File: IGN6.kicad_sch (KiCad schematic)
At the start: 6 parts

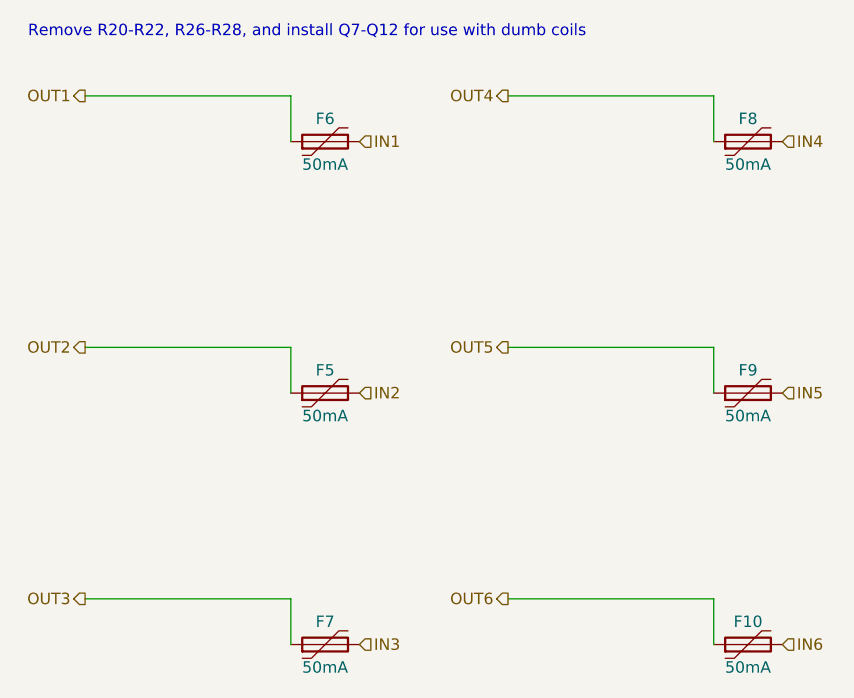
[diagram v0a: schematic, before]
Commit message: test
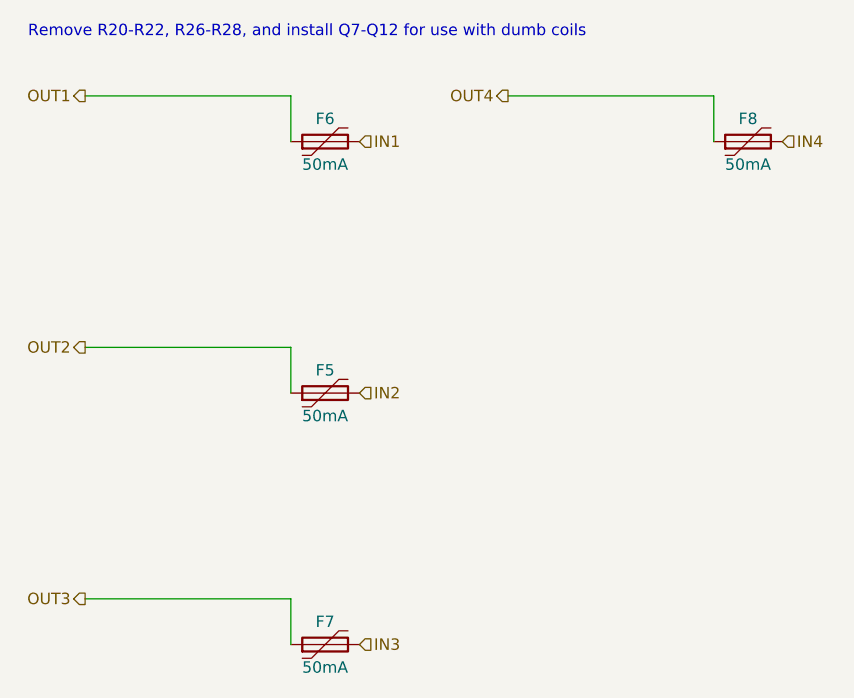
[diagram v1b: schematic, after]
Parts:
- removed F10, F9: 50mA, Fuse:Fuse_0603_1608Metric, symbol Device:Polyfuse
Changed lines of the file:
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@@
-	(wire
-		(pts
-			(xy 160.02 120.65) (xy 182.88 120.65)
-		)
-		(stroke
-			(width 0)
-			(type default)
-		)
-	)
 	(wire
 		(pts
@@
 		(pts
 			(xy 113.03 92.71) (xy 135.89 92.71)
-		)
-		(stroke
-			(width 0)
-			(type default)
-		)
-	)
-	(wire
-		(pts
-			(xy 160.02 92.71) (xy 182.88 92.71)
-		)
-		(stroke
-			(width 0)
-			(type default)
-		)
-	)
-	(wire
-		(pts
-			(xy 182.88 92.71) (xy 182.88 97.79)
-		)
-		(stroke
-			(width 0)
-			(type default)
-		)
-	)
-	(wire
-		(pts
-			(xy 182.88 120.65) (xy 182.88 125.73)
 		)
 		(stroke
@@
 			)
 			(justify left bottom)
-		)
-	)
-	(hierarchical_label "IN5"
-		(shape input)
-		(at 190.5 97.79 0)
-		(fields_autoplaced yes)
-		(effects
-			(font
-				(size 1.27 1.27)
-			)
-			(justify left)
 		)
 	)
@@
 			)
 			(justify left)
-		)
-	)
-	(hierarchical_label "IN6"
-		(shape input)
-		(at 190.5 125.73 0)
-		(fields_autoplaced yes)
-		(effects
-			(font
-				(size 1.27 1.27)
-			)
-			(justify left)
-		)
-	)
-	(hierarchical_label "OUT6"
-		(shape output)
-		(at 160.02 120.65 180)
-		(fields_autoplaced yes)
-		(effects
-			(font
-				(size 1.27 1.27)
-			)
-			(justify right)
-		)
-	)
-	(hierarchical_label "OUT5"
-		(shape output)
-		(at 160.02 92.71 180)
-		(fields_autoplaced yes)
-		(effects
-			(font
-				(size 1.27 1.27)
-			)
-			(justify right)
 		)
 	)
@@
 		)
 	)
-	(symbol
-		(lib_id "Device:Polyfuse")
-		(at 186.69 125.73 90)
-		(unit 1)
-		(exclude_from_sim no)
-		(in_bom yes)
-		(on_board yes)
-		(dnp no)
-		(property "Reference" "F10"
-			(at 186.69 123.19 90)
-			(effects
-				(font
-					(size 1.27 1.27)
-				)
-			)
-		)
-		(property "Value" "50mA"
-			(at 186.69 128.27 90)
-			(effects
-				(font
-					(size 1.27 1.27)
-				)
-			)
-		)
-		(property "Footprint" "Fuse:Fuse_0603_1608Metric"
-			(at 191.77 124.46 0)
-			(effects
-				(font
-					(size 1.27 1.27)
-				)
-				(justify left)
-				(hide yes)
-			)
-		)
-		(property "Datasheet" "~"
-			(at 186.69 125.73 0)
-			(effects
-				(font
-					(size 1.27 1.27)
-				)
-				(hide yes)
-			)
-		)
-		(property "Description" ""
-			(at 186.69 125.73 0)
-			(effects
-				(font
-					(size 1.27 1.27)
-				)
-				(hide yes)
-			)
-		)
-		(property "LCSC" "C369141"
-			(at 186.69 125.73 90)
-			(effects
-				(font
-					(size 1.27 1.27)
-				)
-				(hide yes)
-			)
-		)
-		(pin "1"
-		)
-		(pin "2"
-		)
-		(instances
-			(project "uaefi"
-				(path "/ac264c30-3e9a-4be2-b97a-9949b68bd497/92c4206f-a69e-4d4d-9308-206d3518e11e"
-					(reference "F10")
-					(unit 1)
-				)
-			)
-		)
-	)
-	(symbol
-		(lib_id "Device:Polyfuse")
-		(at 186.69 97.79 90)
-		(unit 1)
-		(exclude_from_sim no)
-		(in_bom yes)
-		(on_board yes)
-		(dnp no)
-		(property "Reference" "F9"
-			(at 186.69 95.25 90)
-			(effects
-				(font
-					(size 1.27 1.27)
-				)
-			)
-		)
-		(property "Value" "50mA"
-			(at 186.69 100.33 90)
-			(effects
-				(font
-					(size 1.27 1.27)
-				)
-			)
-		)
-		(property "Footprint" "Fuse:Fuse_0603_1608Metric"
-			(at 191.77 96.52 0)
-			(effects
-				(font
-					(size 1.27 1.27)
-				)
-				(justify left)
-				(hide yes)
-			)
-		)
-		(property "Datasheet" "~"
-			(at 186.69 97.79 0)
-			(effects
-				(font
-					(size 1.27 1.27)
-				)
-				(hide yes)
-			)
-		)
-		(property "Description" ""
-			(at 186.69 97.79 0)
-			(effects
-				(font
-					(size 1.27 1.27)
-				)
-				(hide yes)
-			)
-		)
-		(property "LCSC" "C369141"
-			(at 186.69 97.79 90)
-			(effects
-				(font
-					(size 1.27 1.27)
-				)
-				(hide yes)
-			)
-		)
-		(pin "1"
-		)
-		(pin "2"
-		)
-		(instances
-			(project "uaefi"
-				(path "/ac264c30-3e9a-4be2-b97a-9949b68bd497/92c4206f-a69e-4d4d-9308-206d3518e11e"
-					(reference "F9")
-					(unit 1)
-				)
-			)
-		)
-	)

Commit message: reset
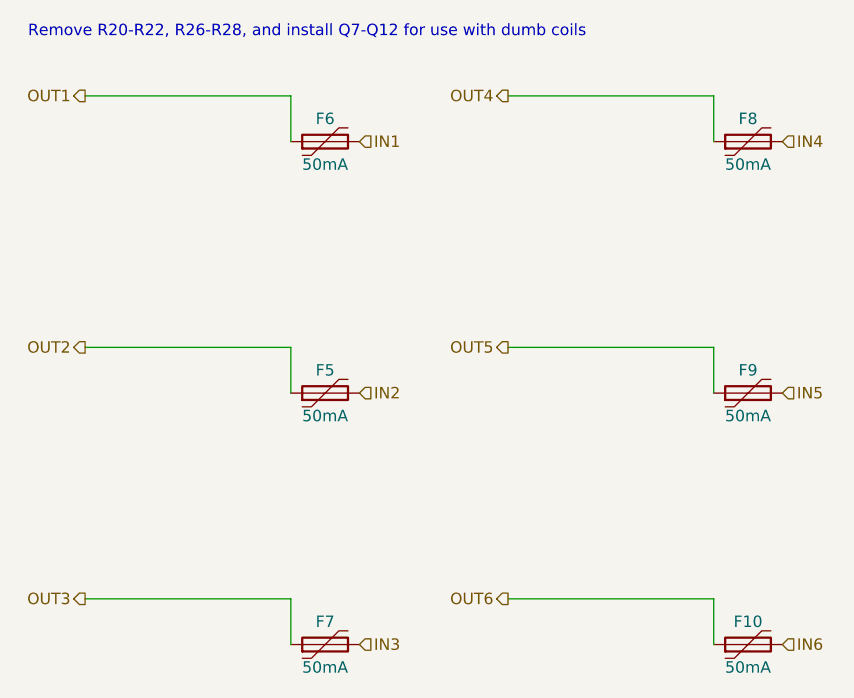
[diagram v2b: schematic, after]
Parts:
- added F10, F9: 50mA, Fuse:Fuse_0603_1608Metric, symbol Device:Polyfuse
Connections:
- new net IN5: F9.2
- new net IN6: F10.2
- new net OUT5: F9.1
- new net OUT6: F10.1
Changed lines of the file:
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@@
+	(wire
+		(pts
+			(xy 160.02 120.65) (xy 182.88 120.65)
+		)
+		(stroke
+			(width 0)
+			(type default)
+		)
+	)
 	(wire
 		(pts
@@
 		(pts
 			(xy 113.03 92.71) (xy 135.89 92.71)
+		)
+		(stroke
+			(width 0)
+			(type default)
+		)
+	)
+	(wire
+		(pts
+			(xy 160.02 92.71) (xy 182.88 92.71)
+		)
+		(stroke
+			(width 0)
+			(type default)
+		)
+	)
+	(wire
+		(pts
+			(xy 182.88 92.71) (xy 182.88 97.79)
+		)
+		(stroke
+			(width 0)
+			(type default)
+		)
+	)
+	(wire
+		(pts
+			(xy 182.88 120.65) (xy 182.88 125.73)
 		)
 		(stroke
@@
 		)
 	)
+	(hierarchical_label "IN5"
+		(shape input)
+		(at 190.5 97.79 0)
+		(fields_autoplaced yes)
+		(effects
+			(font
+				(size 1.27 1.27)
+			)
+			(justify left)
+		)
+	)
 	(hierarchical_label "OUT1"
 		(shape output)
@@
 		)
 	)
+	(hierarchical_label "IN6"
+		(shape input)
+		(at 190.5 125.73 0)
+		(fields_autoplaced yes)
+		(effects
+			(font
+				(size 1.27 1.27)
+			)
+			(justify left)
+		)
+	)
+	(hierarchical_label "OUT6"
+		(shape output)
+		(at 160.02 120.65 180)
+		(fields_autoplaced yes)
+		(effects
+			(font
+				(size 1.27 1.27)
+			)
+			(justify right)
+		)
+	)
+	(hierarchical_label "OUT5"
+		(shape output)
+		(at 160.02 92.71 180)
+		(fields_autoplaced yes)
+		(effects
+			(font
+				(size 1.27 1.27)
+			)
+			(justify right)
+		)
+	)
 	(hierarchical_label "OUT2"
 		(shape output)
@@
 		)
 	)
+	(symbol
+		(lib_id "Device:Polyfuse")
+		(at 186.69 125.73 90)
+		(unit 1)
+		(exclude_from_sim no)
+		(in_bom yes)
+		(on_board yes)
+		(dnp no)
+		(property "Reference" "F10"
+			(at 186.69 123.19 90)
+			(effects
+				(font
+					(size 1.27 1.27)
+				)
+			)
+		)
+		(property "Value" "50mA"
+			(at 186.69 128.27 90)
+			(effects
+				(font
+					(size 1.27 1.27)
+				)
+			)
+		)
+		(property "Footprint" "Fuse:Fuse_0603_1608Metric"
+			(at 191.77 124.46 0)
+			(effects
+				(font
+					(size 1.27 1.27)
+				)
+				(justify left)
+				(hide yes)
+			)
+		)
+		(property "Datasheet" "~"
+			(at 186.69 125.73 0)
+			(effects
+				(font
+					(size 1.27 1.27)
+				)
+				(hide yes)
+			)
+		)
+		(property "Description" ""
+			(at 186.69 125.73 0)
+			(effects
+				(font
+					(size 1.27 1.27)
+				)
+				(hide yes)
+			)
+		)
+		(property "LCSC" "C369141"
+			(at 186.69 125.73 90)
+			(effects
+				(font
+					(size 1.27 1.27)
+				)
+				(hide yes)
+			)
+		)
+		(pin "1"
+		)
+		(pin "2"
+		)
+		(instances
+			(project "uaefi"
+				(path "/ac264c30-3e9a-4be2-b97a-9949b68bd497/92c4206f-a69e-4d4d-9308-206d3518e11e"
+					(reference "F10")
+					(unit 1)
+				)
+			)
+		)
+	)
+	(symbol
+		(lib_id "Device:Polyfuse")
+		(at 186.69 97.79 90)
+		(unit 1)
+		(exclude_from_sim no)
+		(in_bom yes)
+		(on_board yes)
+		(dnp no)
+		(property "Reference" "F9"
+			(at 186.69 95.25 90)
+			(effects
+				(font
+					(size 1.27 1.27)
+				)
+			)
+		)
+		(property "Value" "50mA"
+			(at 186.69 100.33 90)
+			(effects
+				(font
+					(size 1.27 1.27)
+				)
+			)
+		)
+		(property "Footprint" "Fuse:Fuse_0603_1608Metric"
+			(at 191.77 96.52 0)
+			(effects
+				(font
+					(size 1.27 1.27)
+				)
+				(justify left)
+				(hide yes)
+			)
+		)
+		(property "Datasheet" "~"
+			(at 186.69 97.79 0)
+			(effects
+				(font
+					(size 1.27 1.27)
+				)
+				(hide yes)
+			)
+		)
+		(property "Description" ""
+			(at 186.69 97.79 0)
+			(effects
+				(font
+					(size 1.27 1.27)
+				)
+				(hide yes)
+			)
+		)
+		(property "LCSC" "C369141"
+			(at 186.69 97.79 90)
+			(effects
+				(font
+					(size 1.27 1.27)
+				)
+				(hide yes)
+			)
+		)
+		(pin "1"
+		)
+		(pin "2"
+		)
+		(instances
+			(project "uaefi"
+				(path "/ac264c30-3e9a-4be2-b97a-9949b68bd497/92c4206f-a69e-4d4d-9308-206d3518e11e"
+					(reference "F9")
+					(unit 1)
+				)
+			)
+		)
+	)
